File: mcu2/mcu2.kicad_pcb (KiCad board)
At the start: 2 copper layers, 96.7 x 58.3 mm, 36 parts, among them J1 KF128-5.08, J2 Conn_01x30, J8 Conn_01x30, Q1 WSF3085, Q2 PL4009, Q3 PL4009, U1 Pico, U2 motor_driver, U3 max31865_module, U4 dcdc_module

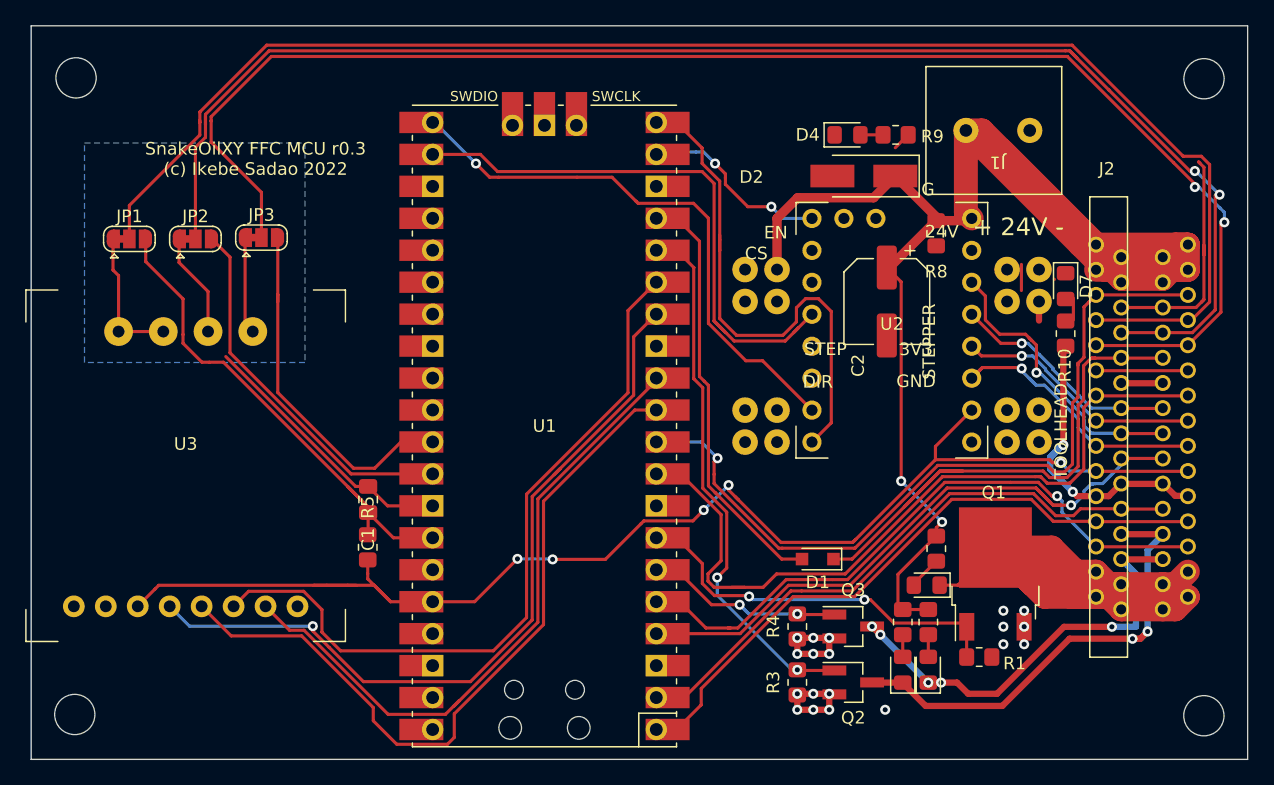
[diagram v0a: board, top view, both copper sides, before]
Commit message: mcu2 gerber
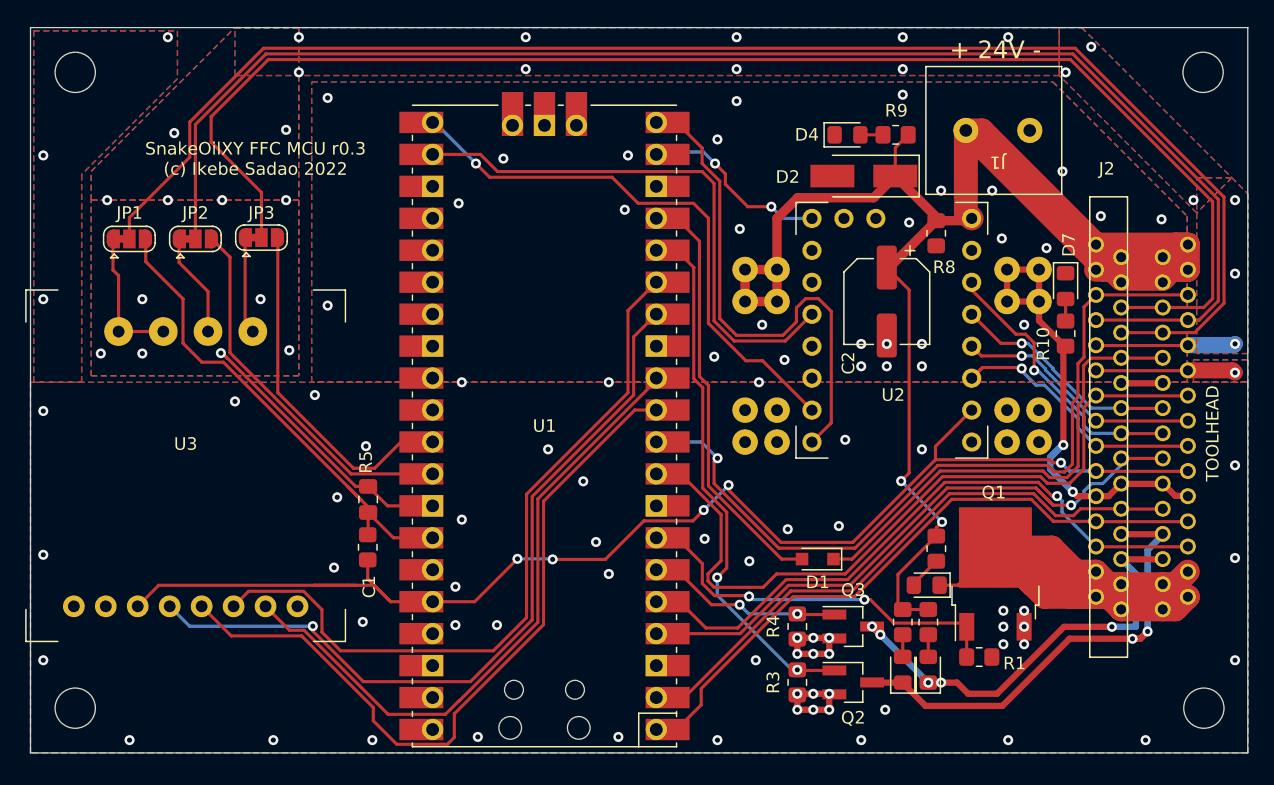
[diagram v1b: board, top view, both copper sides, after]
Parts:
- moved REF** 0.60 mm to (178.4, 141.5)
- moved REF** 0.51 mm to (178.3, 90.9)
- moved REF** 0.50 mm to (88.6, 141.5)
- moved REF** 0.44 mm to (88.6, 90.9)
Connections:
- J2 pad 6: GNDA -> THERM_AUX_2
- J2 pad 7: THERM_0 -> THERM_AUX_1
- J2 pad 8: THERM_AUX_1 -> THERM_0
- J2 pad 9: THERM_AUX_2 -> GNDA
- J8 pad 6: GNDA -> THERM_AUX_2
- J8 pad 7: THERM_0 -> THERM_AUX_1
- J8 pad 8: THERM_AUX_1 -> THERM_0
- J8 pad 9: THERM_AUX_2 -> GNDA
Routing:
- net +5V: track 28.0 -> 38.5 mm
- net GNDA: track 40.5 -> 33.0 mm, vias 0 -> 27
- net PROBE_ZMIN_24V: track 43.7 -> 37.7 mm
- net THERM_AUX_2: track 118.1 -> 112.7 mm, vias 2 -> 0
- net PART_FAN_CTRL: track 19.2 -> 13.9 mm
- net ADXL345_CS: track 49.6 -> 45.7 mm
- net ADXL345_SDO: track 53.4 -> 49.7 mm
- net SERVO_NEOPIXEL: track 61.9 -> 58.3 mm
- net GND: track 26.4 -> 29.5 mm, vias 19 -> 90
- net AUX2: track 28.6 -> 25.5 mm
- net E_DIR: track 42.5 -> 39.7 mm
- net STEPPER_A2: track 23.9 -> 21.6 mm
- net ADXL345_SDA: track 50.8 -> 48.7 mm
- net HEATER_CTRL: track 30.9 -> 28.9 mm
- net E_CS: track 45.4 -> 43.6 mm
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- added copper zone on B.Cu, net GND
- added copper zone on F.Cu, net GND
- added copper zone on F.Cu, net GNDA
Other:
- board size 96.7 x 58.3 mm -> 96.8 x 57.7 mm
- board text removed: "24V"
- board text removed: "3V3"
- board text removed: "CS"
- board text removed: "DIR"
- board text removed: "EN"
- board text removed: "G"
- board text removed: "GND"
- board text removed: "STEP"
- board text removed: "STEPPER"
